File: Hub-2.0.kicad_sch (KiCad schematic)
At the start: 5 parts, among them CN1 DT15-12PA, CN2 DT15-12PA, SW1 SW_Push_Open, SW2 SW_Push_Open

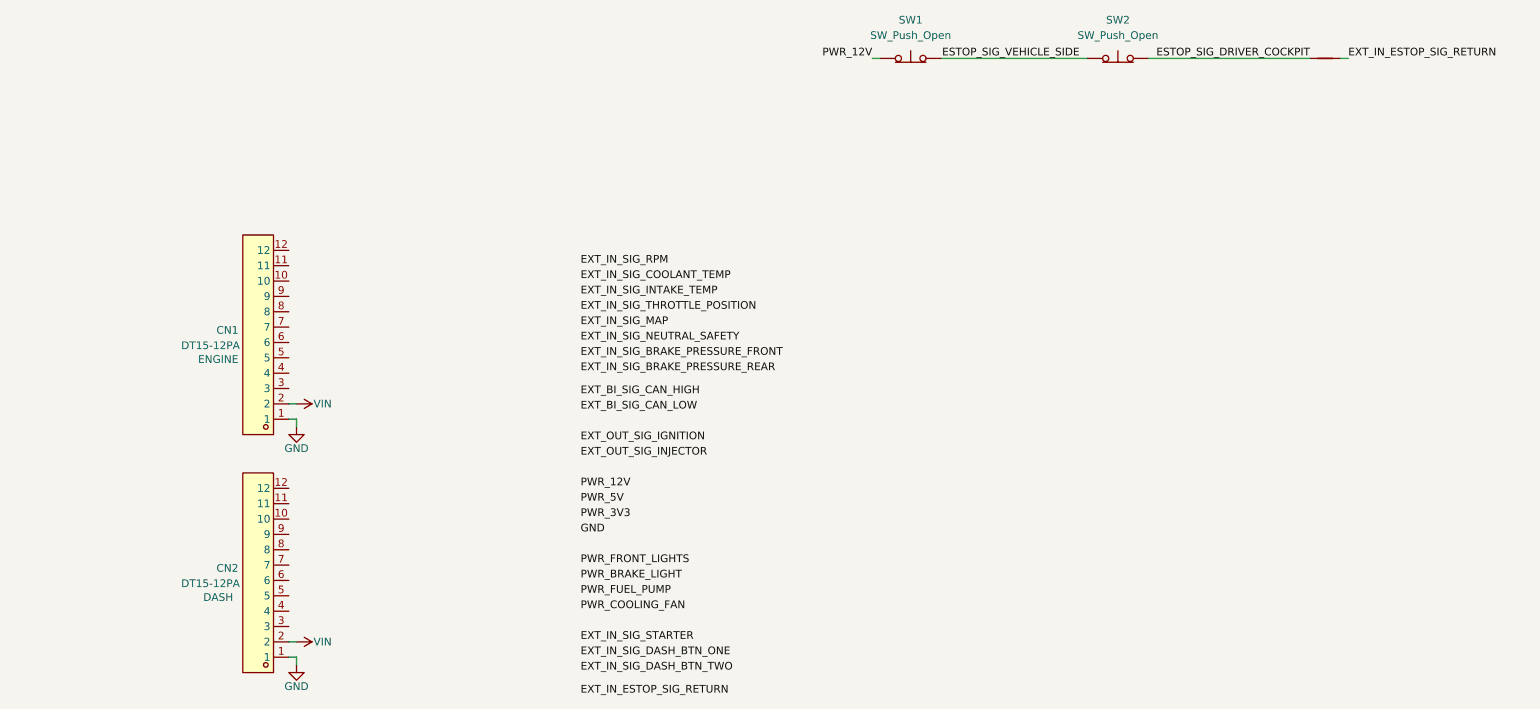
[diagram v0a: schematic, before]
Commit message: SCH Save
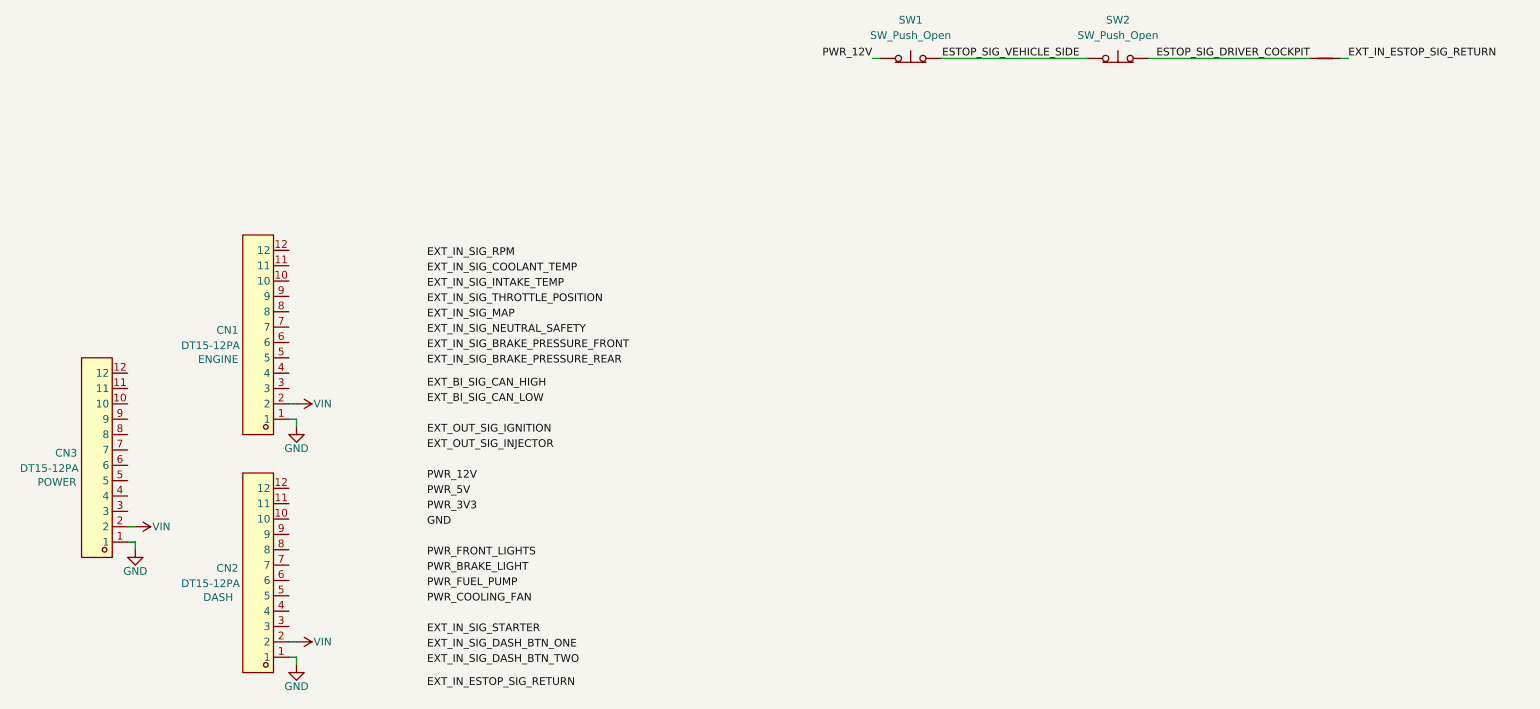
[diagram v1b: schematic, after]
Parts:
- added CN3: DT15-12PA, EasyEDA:CONN-TH_DT15-12PA, symbol EasyEDA:DT15-12PA
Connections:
- net GND: now also CN3.1
- net VIN: now also CN3.2
